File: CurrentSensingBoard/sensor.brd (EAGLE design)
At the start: 54 x 78 mm, 13 parts, among them U1 MAX11634EEE+T21-0055H_16-L

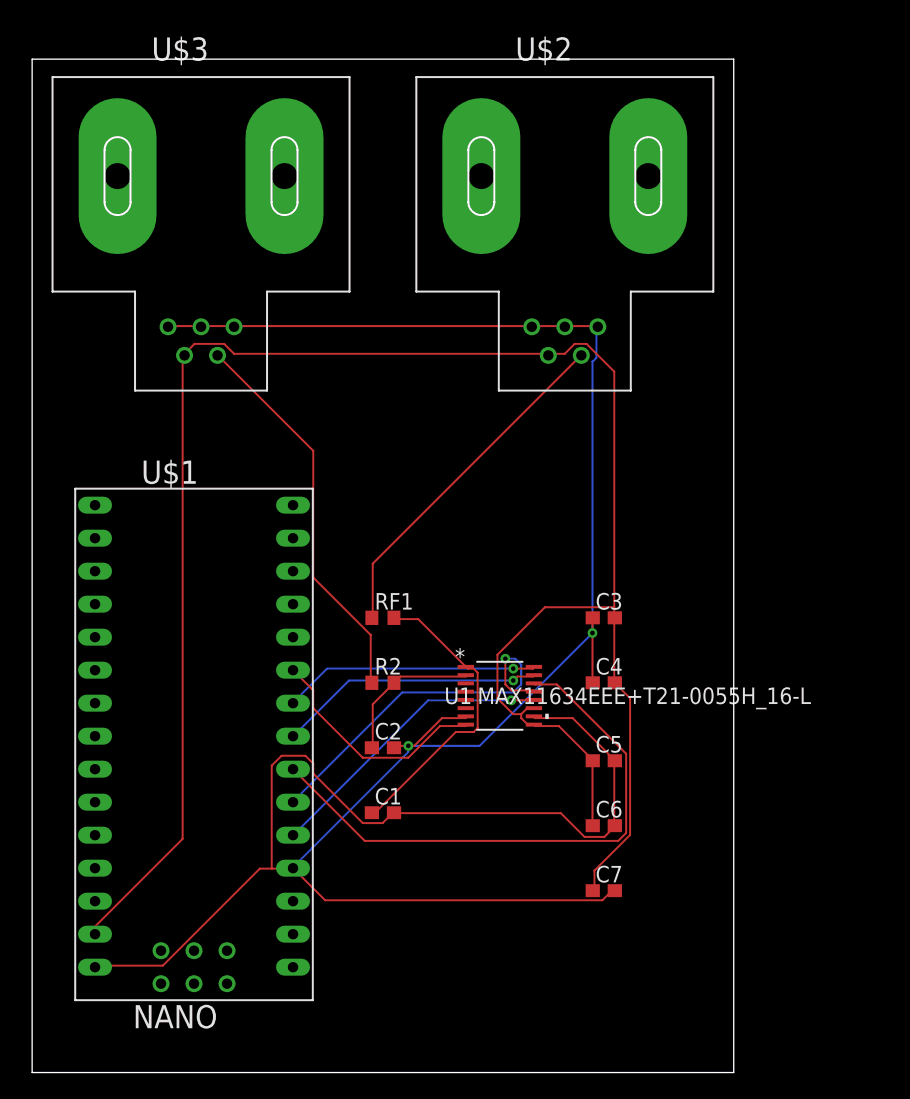
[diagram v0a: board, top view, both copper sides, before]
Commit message: compacted board
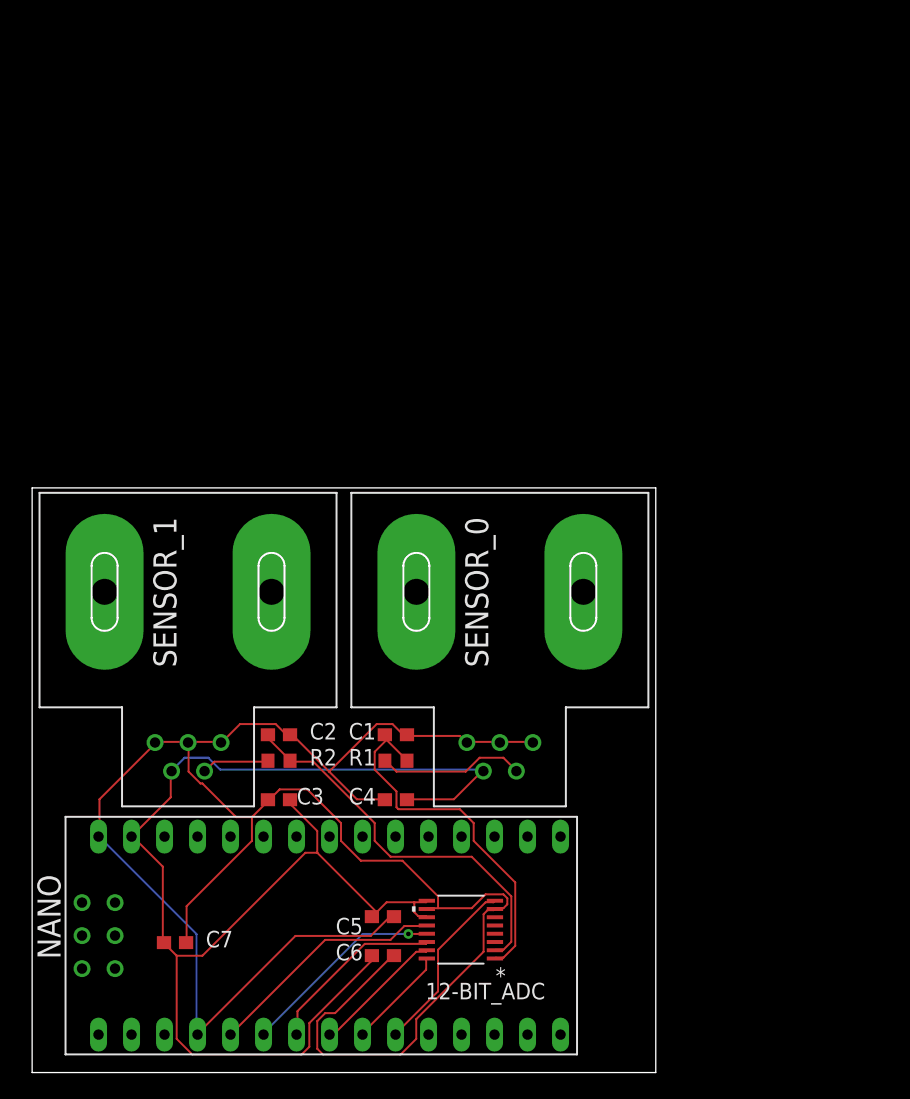
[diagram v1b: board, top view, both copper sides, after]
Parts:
- removed RF1: RF0, rcl:R0603
- removed U$2, U$3: CQ2065, CurrentSensing:CQ2065
- removed U1: MAX11634EEE+T21-0055H_16-L, CurrentSensing:21-0055H_16-L
- added 12-BIT_ADC: MAX11634EEE+T21-0055H_16-L, CurrentSensing:21-0055H_16-L
- added R1: RF0, rcl:R0603
- added SENSOR_0, SENSOR_1: CQ2065, CurrentSensing:CQ2065
- moved C7 33.2 mm to (11.0, 10.0)
- moved C3 28.7 mm to (19.0, 21.0)
- moved C5 20.8 mm to (27.0, 12.0)
- moved C6 19.7 mm to (27.0, 9.00)
- moved C4 18.4 mm to (28.0, 21.0)
- moved R2 10.0 mm to (19.0, 24.0)
- moved U$1 9.06 mm to (14.0, 8.00), turned to 270 degrees
- moved C2 8.06 mm to (19.0, 26.0)
- moved C1 6.08 mm to (28.0, 26.0)
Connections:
- new net N$1: U$1.TX0
- new net TX_TEENSY: U$1.RX1
- net !CNVST!: now also 12-BIT_ADC.8; no longer U1.8
- net !CS!: now also 12-BIT_ADC.12; no longer U1.12
- net !EOC!: now also 12-BIT_ADC.16; no longer U1.16
- net +5V: now also 12-BIT_ADC.11, 12-BIT_ADC.9, SENSOR_0.2, SENSOR_1.2; no longer U$2.2, U$3.2, U1.11, U1.9
- net AIN0: now also 12-BIT_ADC.1, R1.2; no longer RF1.2, U1.1
- net AIN1: now also 12-BIT_ADC.2; no longer U1.2
- net DIN: now also 12-BIT_ADC.14; no longer U1.14
- net DOUT: now also 12-BIT_ADC.15; no longer U1.15
- net GND: now also 12-BIT_ADC.10, 12-BIT_ADC.7, SENSOR_0.1, SENSOR_0.3, SENSOR_0.5, SENSOR_1.1, SENSOR_1.3, SENSOR_1.5; no longer U$2.1, U$2.3, U$2.5, U$3.1, U$3.3, U$3.5, U1.10, U1.7
- net N$3: now also SENSOR_1.4; no longer U$3.4
- net N$5: now also R1.1, SENSOR_0.4; no longer RF1.1, U$2.4
- net SCLK: now also 12-BIT_ADC.13; no longer U1.13
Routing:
- net +5V: track 153.9 -> 107.7 mm
- net GND: track 195.6 -> 165.3 mm, vias 2 -> 0
- net DIN: track 43.6 -> 14.0 mm
- net N$3: track 30.2 -> 5.24 mm
- net AIN1: track 11.5 -> 29.9 mm
- net N$5: track 26.9 -> 11.3 mm
- net SCLK: track 28.7 -> 15.8 mm
- net !EOC!: track 19.7 -> 7.89 mm, vias 1 -> 0
- net DOUT: track 20.5 -> 10.2 mm, vias 1 -> 0
- net AIN0: track 23.3 -> 28.6 mm
- net !CS!: track 22.8 -> 18.6 mm, vias 1 -> 0
- net !CNVST!: track 18.0 -> 13.8 mm
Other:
- board size 54 x 78 mm -> 48 x 45 mm

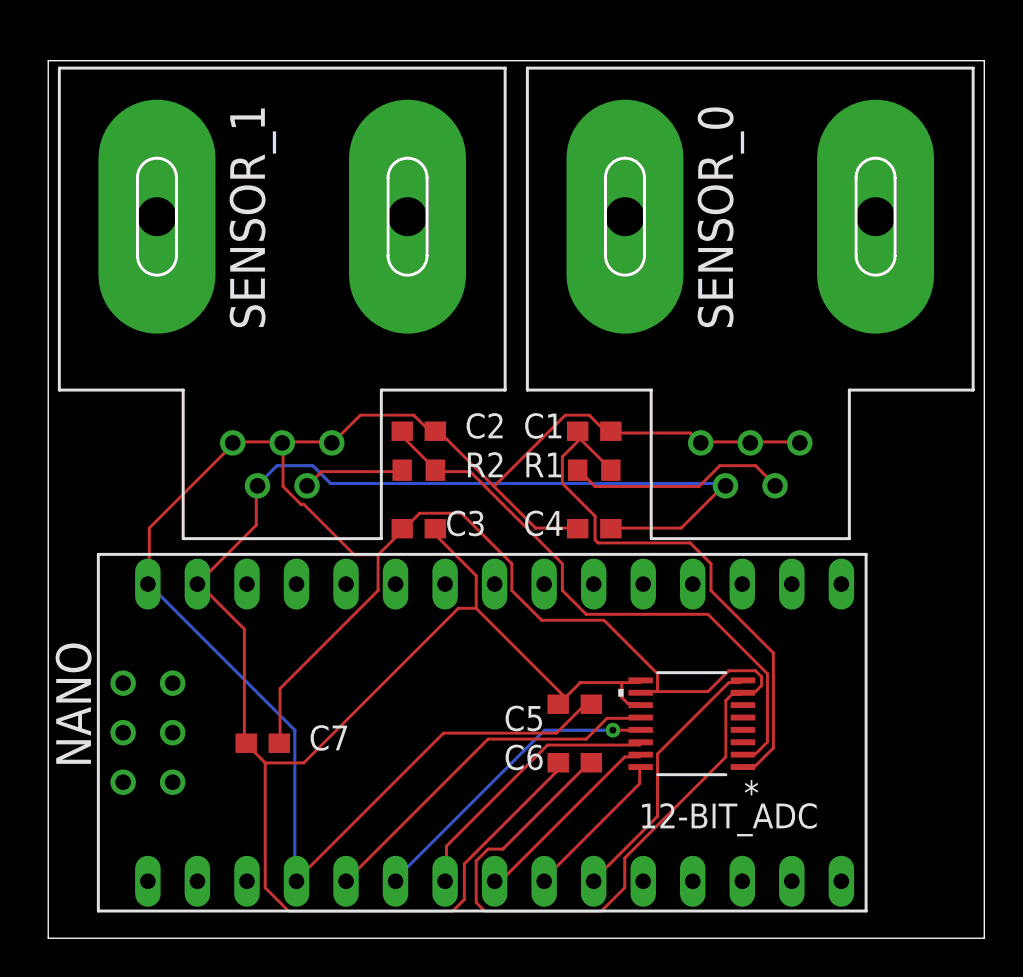
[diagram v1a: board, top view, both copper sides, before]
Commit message: implmented ground plane
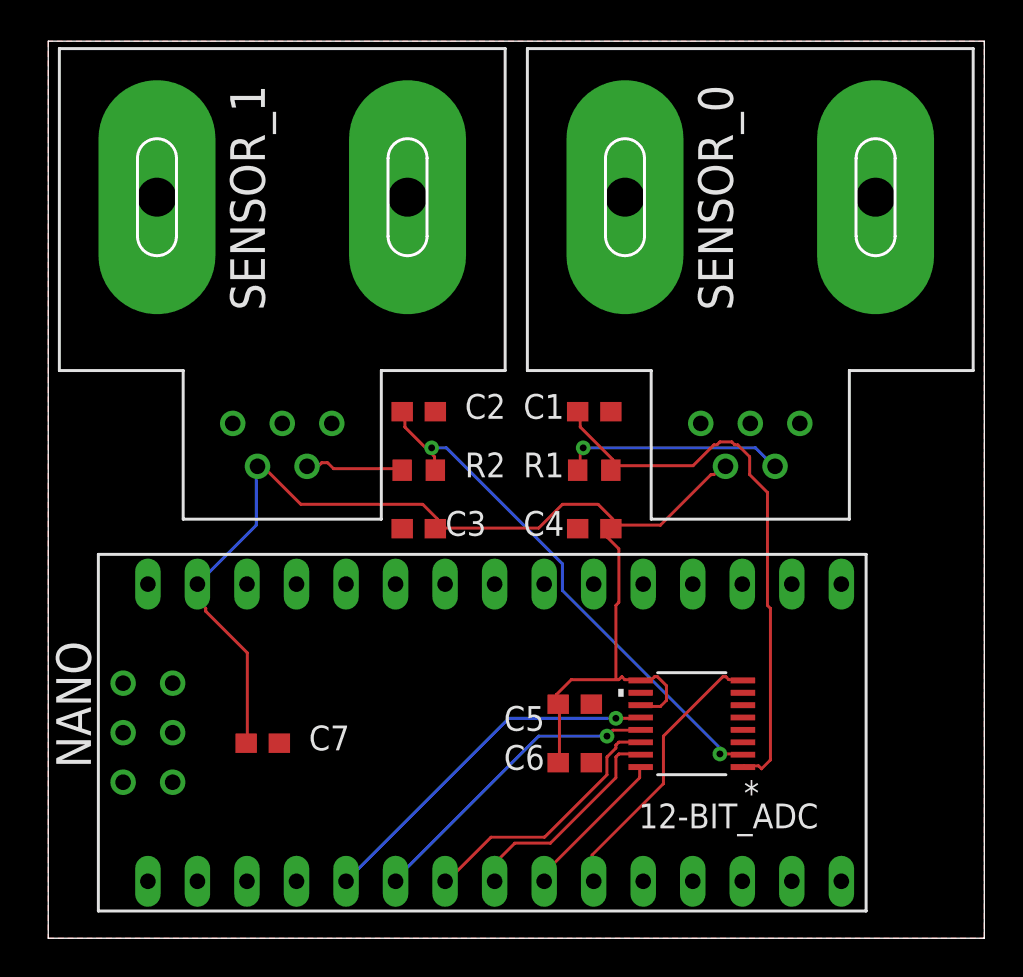
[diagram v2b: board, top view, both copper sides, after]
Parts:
- moved C1 1.00 mm to (28.0, 27.0)
- moved C2 1.00 mm to (19.0, 27.0)
- moved SENSOR_0 1.00 mm to (36.0, 38.0)
- moved SENSOR_1 1.00 mm to (12.0, 38.0)
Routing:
- net GND: track 165.3 -> 0.00 mm
- net +5V: track 107.7 -> 65.4 mm
- net AIN1: track 29.9 -> 27.4 mm, vias 0 -> 2
- net DOUT: track 10.2 -> 11.4 mm
- net AIN0: track 28.6 -> 29.6 mm
- net !CNVST!: track 13.8 -> 14.4 mm
- net N$5: track 11.3 -> 11.5 mm, vias 0 -> 1
- net !CS!: vias 0 -> 1
- added copper zone on layer 1, net GND
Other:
- board size 48 x 45 mm -> 48 x 46 mm

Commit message: implemented connector
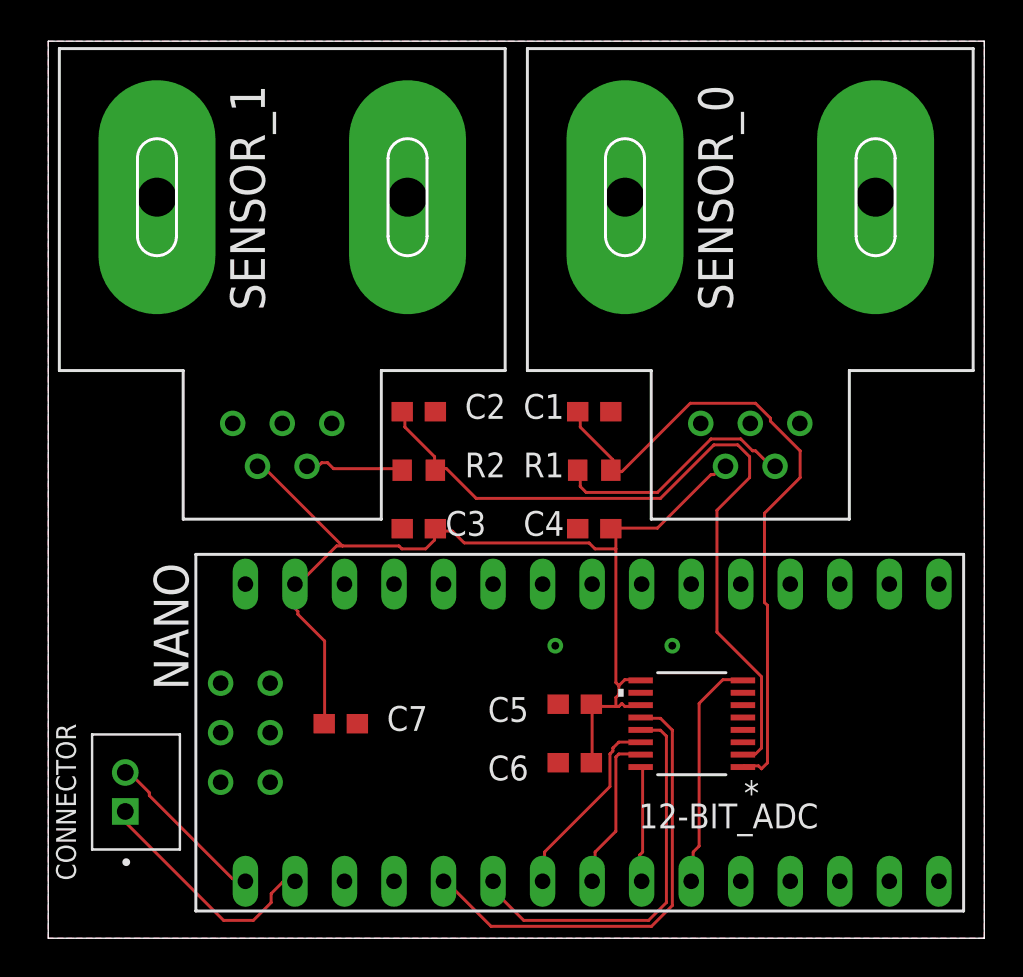
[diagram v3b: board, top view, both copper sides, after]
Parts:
- added CONNECTOR: B2B-PH-K-S(LF)(SN), B2B-PH-K-S_LF__SN_:JST_B2B-PH-K-S(LF)(SN)
- moved U$1 5.00 mm to (19.0, 8.00)
- moved C7 4.12 mm to (15.0, 11.0)
- turned C5 to 180 degrees
- turned C6 to 180 degrees
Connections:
- removed net N$1: U$1.TX0
- new net RX_TEENSY: CONNECTOR.2, U$1.TX0
- net TX_TEENSY: now also CONNECTOR.1
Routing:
- net TX_TEENSY: track 0.00 -> 12.4 mm
- net AIN1: track 27.4 -> 39.6 mm, vias 2 -> 0
- net +5V: track 65.4 -> 56.0 mm
- net RX_TEENSY: track 0.00 -> 8.65 mm
- net !CS!: track 18.6 -> 24.0 mm, vias 1 -> 0
- net AIN0: track 29.6 -> 34.4 mm
- net SCLK: track 15.8 -> 20.3 mm, vias 1 -> 0
- net DIN: track 13.6 -> 9.87 mm
- net DOUT: track 11.4 -> 8.23 mm
- net !CNVST!: track 14.4 -> 12.0 mm
- net !EOC!: track 7.89 -> 6.00 mm
- net N$5: track 11.5 -> 12.9 mm, vias 1 -> 0
- added copper zone on layer 16, net GND
